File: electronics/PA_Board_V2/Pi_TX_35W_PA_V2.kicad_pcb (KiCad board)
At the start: 4 copper layers, 100 x 100 mm, 183 parts, among them J1 Conn_Coaxial, J10 Conn_01x05, J2 Conn_01x04, J3 Conn_01x05, J4 Conn_01x02, J5 Conn_Coaxial, J6 Conn_01x06, J7 Conn_Coaxial, J8 Conn_Coaxial, J9 USB_B_Micro, K1 G6E, Q1 AOD4185, Q2 BC848W, SW1 SW_Push, U1 PSA4-5043+, U10 INA219AxD, U11 TLV70233, U12 LM2904, U13 ATSAMD21E18A-A, U14 Directional_Coupler, U15 74LV1T34, U2 LM75B, U3 PSA4-5043+, U4 RA35H1516M, U5 74LV1T34, U6 LMR51420, U7 MCP4725, U8 TPS22810DBV, U9 AP2204K-ADJ

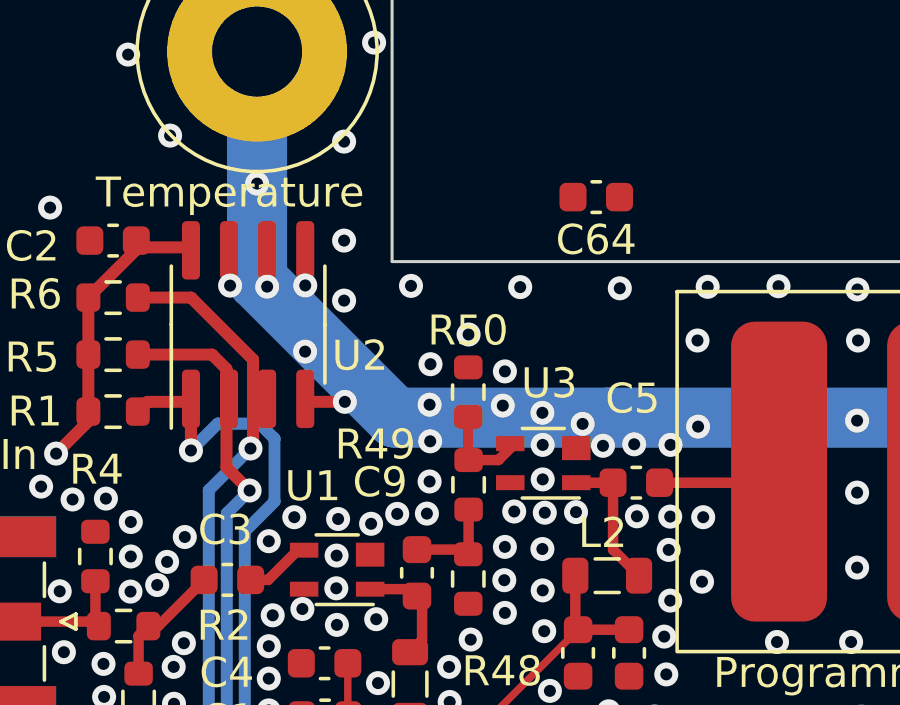
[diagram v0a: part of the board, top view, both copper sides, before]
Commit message: Save unlocked Kicad files for PA Board V2
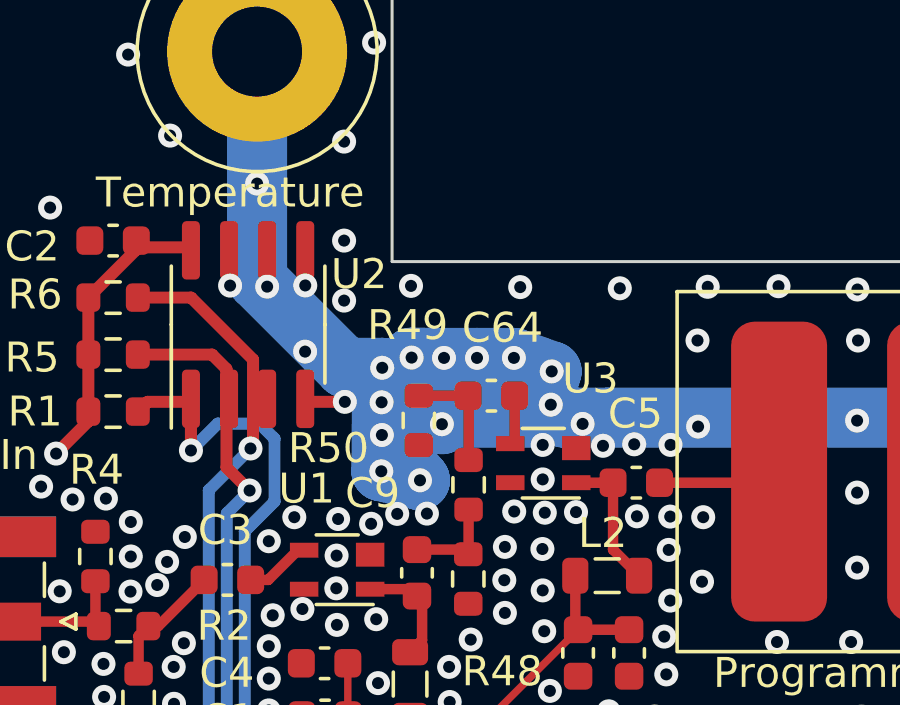
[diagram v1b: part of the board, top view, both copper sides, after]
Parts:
- moved C64 7.49 mm to (118.8, 77.5)
- moved R50 1.90 mm to (116.4, 78.3), turned to -90 degrees
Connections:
- R22 pad 2: Net-(U14-Fterm) -> Net-(D2-K)
- R23 pad 2: Net-(U14-Fterm) -> Net-(D2-K)
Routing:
- net GND: track 256.4 -> 275.1 mm, vias 415 -> 419
- net Net-(C64-Pad2): track 0.00 -> 3.81 mm
- net (no net): track 3.21 -> 0.00 mm
- net Net-(C64-Pad1): track 0.00 -> 1.66 mm
